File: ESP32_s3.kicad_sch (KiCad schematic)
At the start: 74 parts, among them J1 Conn_01x02_Pin, J11 backup, J12 Conn_01x02_Pin, J13 Jetson Power Supply, J14 TXRX, J15 TXRX2, J2 programming header usb, J3 Conn_01x02, J4 Servo motor, J5 PJ-040DH, J7 Conn_01x02, J8 Conn_01x02, J9 Conn_01x02, Q1 BSS138, SW1 SW_Push, SW2 SW_Push, U1 ESP32-S3-WROOM-1-N8R2, U2 LM1117T-ADJ, U3 L298N, U4 TPS61088RHLR, Y1 Crystal

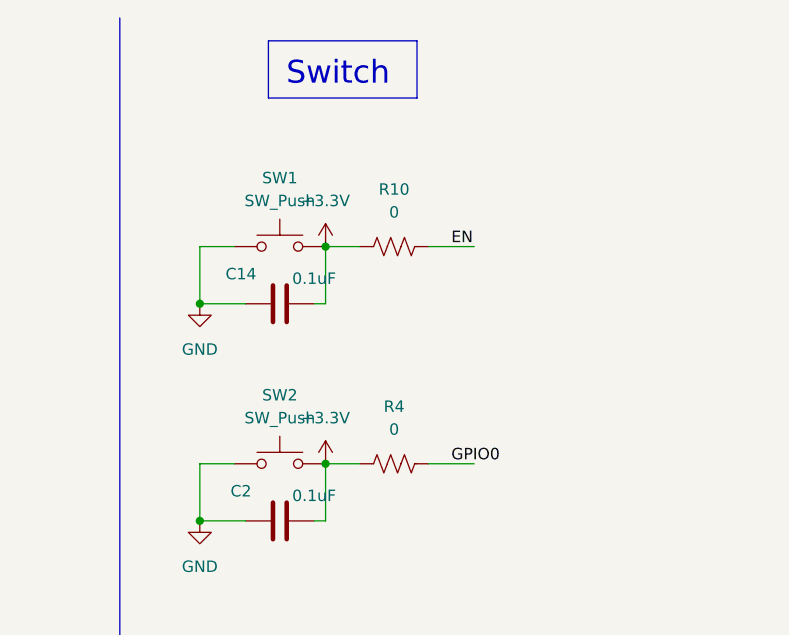
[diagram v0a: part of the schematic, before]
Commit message: update PCB layout
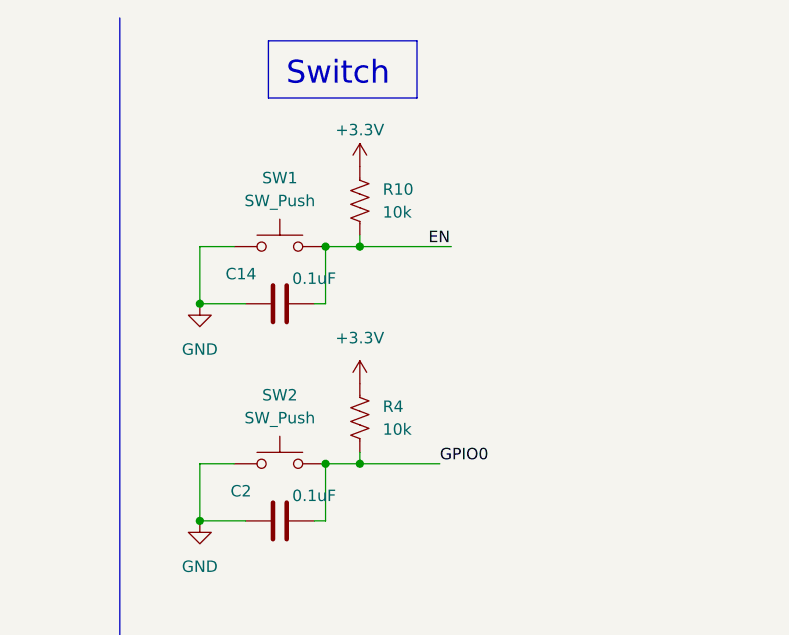
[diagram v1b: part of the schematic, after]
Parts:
- R10, R4: value 0 -> 10k; footprint RMCF1206ZR0R00:RESC3216X70N -> CRCW080535K7FKEA:RESC2012X50N
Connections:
- net +3.3V: now also R10.2, R4.2; no longer C14.1, C2.1, R10.1, R4.1, SW1.2, SW2.2
- net EN: now also C14.1, R10.1, SW1.2; no longer R10.2
- net GPIO0: now also C2.1, R4.1, SW2.2; no longer R4.2
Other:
- moved on the sheet: R10, R4
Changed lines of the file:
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@@
 	)
 	(junction
+		(at 361.95 36.83)
+		(diameter 0)
+		(color 0 0 0 0)
+	)
+	(junction
 		(at 289.56 67.31)
 		(diameter 0)
@@
 	)
 	(junction
+		(at 361.95 60.96)
+		(diameter 0)
+		(color 0 0 0 0)
+	)
+	(junction
 		(at 204.47 97.79)
 		(diameter 0)
@@
 	(wire
 		(pts
-			(xy 358.14 60.96) (xy 361.95 60.96)
-		)
-		(stroke
-			(width 0)
-			(type default)
-		)
-	)
-	(wire
-		(pts
 			(xy 369.57 224.79) (xy 364.49 224.79)
 		)
@@
 	(wire
 		(pts
+			(xy 361.95 59.69) (xy 361.95 60.96)
+		)
+		(stroke
+			(width 0)
+			(type default)
+		)
+	)
+	(wire
+		(pts
 			(xy 224.79 36.83) (xy 213.36 36.83)
 		)
@@
 	(wire
 		(pts
+			(xy 361.95 35.56) (xy 361.95 36.83)
+		)
+		(stroke
+			(width 0)
+			(type default)
+		)
+	)
+	(wire
+		(pts
 			(xy 50.8 229.87) (xy 50.8 226.06)
 		)
@@
 	(wire
 		(pts
+			(xy 361.95 60.96) (xy 370.84 60.96)
+		)
+		(stroke
+			(width 0)
+			(type default)
+		)
+	)
+	(wire
+		(pts
 			(xy 58.42 226.06) (xy 66.04 226.06)
 		)
@@
 	(wire
 		(pts
-			(xy 369.57 60.96) (xy 374.65 60.96)
-		)
-		(stroke
-			(width 0)
-			(type default)
-		)
-	)
-	(wire
-		(pts
 			(xy 80.01 49.53) (xy 68.58 49.53)
 		)
@@
 	(wire
 		(pts
+			(xy 361.95 60.96) (xy 358.14 60.96)
+		)
+		(stroke
+			(width 0)
+			(type default)
+		)
+	)
+	(wire
+		(pts
 			(xy 359.41 208.28) (xy 350.52 208.28)
 		)
@@
 	(wire
 		(pts
+			(xy 361.95 36.83) (xy 372.11 36.83)
+		)
+		(stroke
+			(width 0)
+			(type default)
+		)
+	)
+	(wire
+		(pts
 			(xy 146.05 97.79) (xy 158.75 97.79)
 		)
@@
 	(wire
 		(pts
-			(xy 369.57 36.83) (xy 374.65 36.83)
-		)
-		(stroke
-			(width 0)
-			(type default)
-		)
-	)
-	(wire
-		(pts
 			(xy 275.59 67.31) (xy 260.35 67.31)
 		)
@@
 	)
 	(label "EN"
-		(at 372.11 36.83 0)
+		(at 369.57 36.83 0)
 		(fields_autoplaced yes)
 		(effects
@@
 	)
 	(label "GPIO0"
-		(at 372.11 60.96 0)
+		(at 370.84 60.96 0)
 		(fields_autoplaced yes)
 		(effects
@@
 	(symbol
 		(lib_id "Device:R_US")
-		(at 365.76 36.83 90)
+		(at 361.95 31.75 180)
 		(unit 1)
 		(exclude_from_sim no)
@@
 		(fields_autoplaced yes)
 		(property "Reference" "R10"
-			(at 365.76 30.48 90)
+			(at 364.49 30.4799 0)
 			(effects
 				(font
 					(size 1.27 1.27)
 				)
+				(justify right)
 			)
 		)
-		(property "Value" "0"
-			(at 365.76 33.02 90)
+		(property "Value" "10k"
+			(at 364.49 33.0199 0)
 			(effects
 				(font
 					(size 1.27 1.27)
 				)
+				(justify right)
 			)
 		)
-		(property "Footprint" "RMCF1206ZR0R00:RESC3216X70N"
-			(at 366.014 35.814 90)
+		(property "Footprint" "CRCW080535K7FKEA:RESC2012X50N"
+			(at 360.934 31.496 90)
 			(effects
 				(font
@@
 		)
 		(property "Datasheet" "https://www.seielect.com/catalog/sei-rmcf_rmcp.pdf"
-			(at 365.76 36.83 0)
+			(at 361.95 31.75 0)
 			(effects
 				(font
@@
 		)
 		(property "Description" "Resistor, US symbol"
-			(at 365.76 36.83 0)
+			(at 361.95 31.75 0)
 			(effects
 				(font
@@
 	(symbol
 		(lib_id "Device:R_US")
-		(at 365.76 60.96 90)
+		(at 361.95 55.88 180)
 		(unit 1)
 		(exclude_from_sim no)
@@
 		(fields_autoplaced yes)
 		(property "Reference" "R4"
-			(at 365.76 54.61 90)
+			(at 364.49 54.6099 0)
 			(effects
 				(font
 					(size 1.27 1.27)
 				)
+				(justify right)
 			)
 		)
-		(property "Value" "0"
-			(at 365.76 57.15 90)
+		(property "Value" "10k"
+			(at 364.49 57.1499 0)
 			(effects
 				(font
 					(size 1.27 1.27)
 				)
+				(justify right)
 			)
 		)
-		(property "Footprint" "RMCF1206ZR0R00:RESC3216X70N"
-			(at 366.014 59.944 90)
+		(property "Footprint" "CRCW080535K7FKEA:RESC2012X50N"
+			(at 360.934 55.626 90)
 			(effects
 				(font
@@
 		)
 		(property "Datasheet" "https://www.seielect.com/catalog/sei-rmcf_rmcp.pdf"
-			(at 365.76 60.96 0)
+			(at 361.95 55.88 0)
 			(effects
 				(font
@@
 		)
 		(property "Description" "Resistor, US symbol"
-			(at 365.76 60.96 0)
+			(at 361.95 55.88 0)
 			(effects
 				(font
@@
 		(lib_name "+3.3V_2")
 		(lib_id "power:+3.3V")
-		(at 358.14 36.83 0)
+		(at 361.95 27.94 0)
 		(unit 1)
 		(exclude_from_sim no)
@@
 		(on_board yes)
 		(dnp no)
-		(fields_autoplaced yes)
 		(property "Reference" "#PWR028"
-			(at 358.14 40.64 0)
+			(at 361.95 31.75 0)
 			(effects
 				(font
@@
 		)
 		(property "Value" "+3.3V"
-			(at 358.14 31.75 0)
+			(at 361.95 23.876 0)
 			(effects
 				(font
@@
 		)
 		(property "Footprint" ""
-			(at 358.14 36.83 0)
+			(at 361.95 27.94 0)
 			(effects
 				(font
@@
 		)
 		(property "Datasheet" ""
-			(at 358.14 36.83 0)
+			(at 361.95 27.94 0)
 			(effects
 				(font
@@
 		)
 		(property "Description" "Power symbol creates a global label with name \"+3.3V\""
-			(at 358.14 36.83 0)
+			(at 361.95 27.94 0)
 			(effects
 				(font
@@
 		(lib_name "+3.3V_2")
 		(lib_id "power:+3.3V")
-		(at 358.14 60.96 0)
+		(at 361.95 52.07 0)
 		(unit 1)
 		(exclude_from_sim no)
@@
 		(fields_autoplaced yes)
 		(property "Reference" "#PWR027"
-			(at 358.14 64.77 0)
+			(at 361.95 55.88 0)
 			(effects
 				(font
@@
 		)
 		(property "Value" "+3.3V"
-			(at 358.14 55.88 0)
+			(at 361.95 46.99 0)
 			(effects
 				(font
@@
 		)
 		(property "Footprint" ""
-			(at 358.14 60.96 0)
+			(at 361.95 52.07 0)
 			(effects
 				(font
@@
 		)
 		(property "Datasheet" ""
-			(at 358.14 60.96 0)
+			(at 361.95 52.07 0)
 			(effects
 				(font
@@
 		)
 		(property "Description" "Power symbol creates a global label with name \"+3.3V\""
-			(at 358.14 60.96 0)
+			(at 361.95 52.07 0)
 			(effects
 				(font
